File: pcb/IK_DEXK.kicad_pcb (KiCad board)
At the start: 2 copper layers, 70 x 76 mm, 11 parts, among them SW1 SW_Push, SW2 SW_Push, SW3 SW_Push, SW4 SW_Push, SW5 SW_Push, SW6 SW_Push, SW7 SW_Push, SW8 SW_Push, SW9 SW_Push, U1 MOUDLE-SEEEDUINO-XIAO, U2 ER_OLEDM0.91_1x-I2C

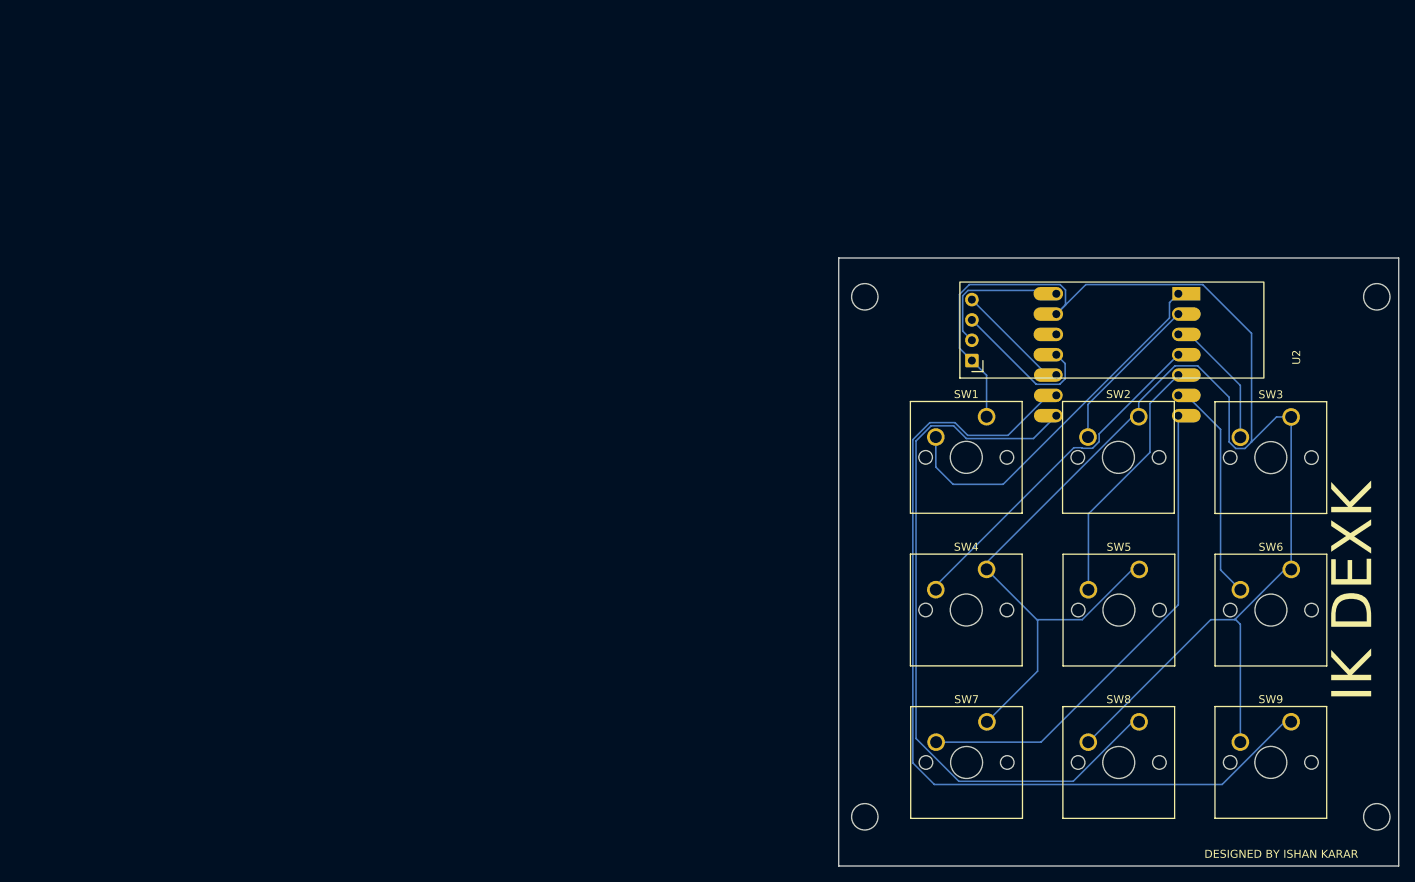
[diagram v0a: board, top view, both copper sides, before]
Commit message: everything
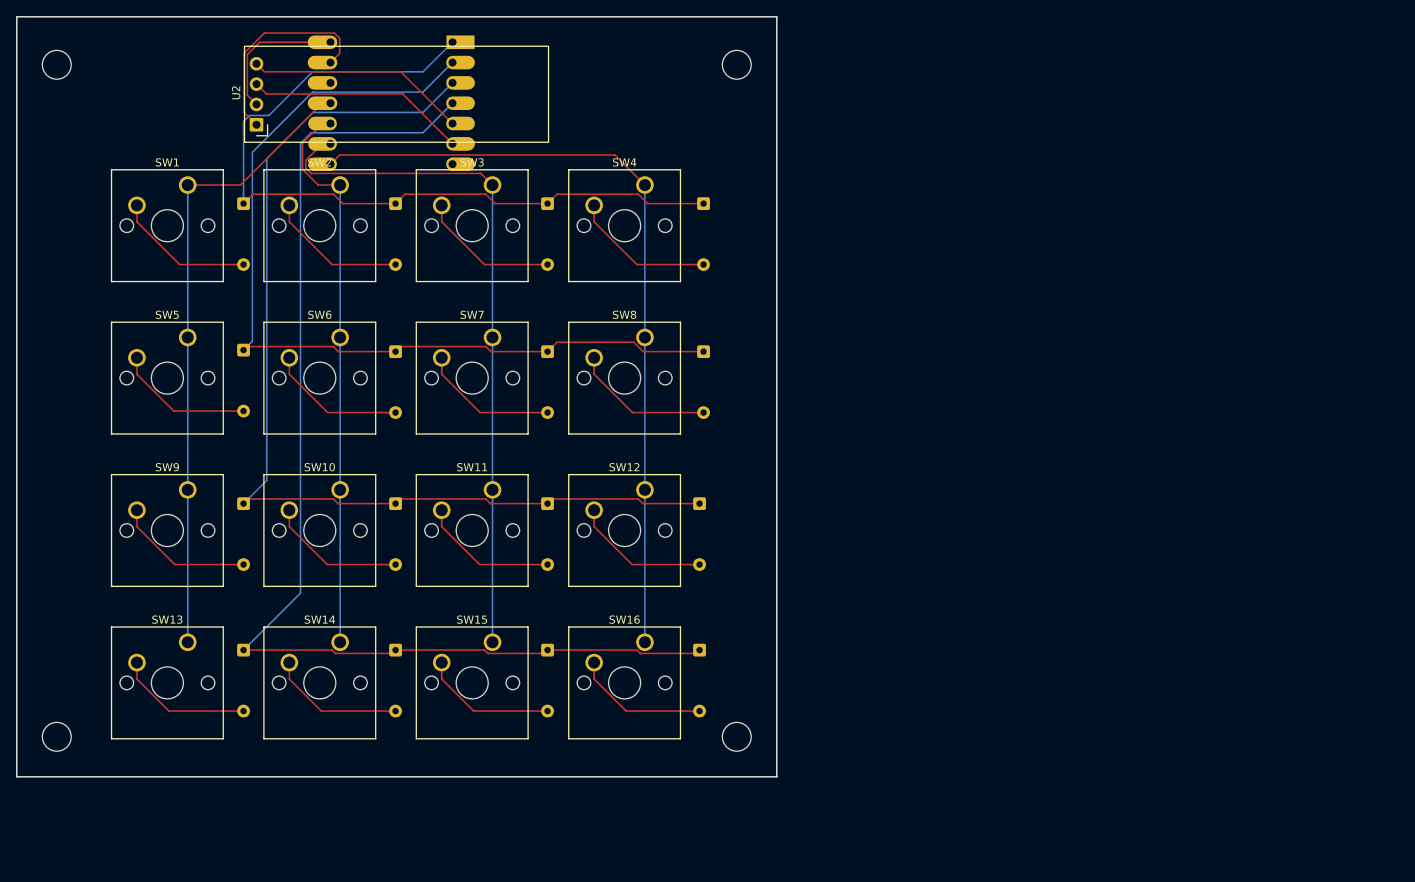
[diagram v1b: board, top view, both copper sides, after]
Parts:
- added D1: 1N4148, Diode_THT:D_DO-35_SOD27_P7.62mm_Horizontal, B.Cu at (28.3, 23.4)
- added D10: 1N4148, Diode_THT:D_DO-35_SOD27_P7.62mm_Horizontal, B.Cu at (47.3, 60.9)
- added D11: 1N4148, Diode_THT:D_DO-35_SOD27_P7.62mm_Horizontal, B.Cu at (66.3, 60.9)
- added D12: 1N4148, Diode_THT:D_DO-35_SOD27_P7.62mm_Horizontal, B.Cu at (85.3, 60.9)
- added D13: 1N4148, Diode_THT:D_DO-35_SOD27_P7.62mm_Horizontal, B.Cu at (28.3, 79.2)
- added D14: 1N4148, Diode_THT:D_DO-35_SOD27_P7.62mm_Horizontal, B.Cu at (47.3, 79.2)
- added D15: 1N4148, Diode_THT:D_DO-35_SOD27_P7.62mm_Horizontal, B.Cu at (66.3, 79.2)
- added D16: 1N4148, Diode_THT:D_DO-35_SOD27_P7.62mm_Horizontal, B.Cu at (85.3, 79.2)
- added D2: 1N4148, Diode_THT:D_DO-35_SOD27_P7.62mm_Horizontal, B.Cu at (47.3, 23.4)
- added D3: 1N4148, Diode_THT:D_DO-35_SOD27_P7.62mm_Horizontal, B.Cu at (66.3, 23.4)
- added D4: 1N4148, Diode_THT:D_DO-35_SOD27_P7.62mm_Horizontal, B.Cu at (85.8, 23.4)
- added D5: 1N4148, Diode_THT:D_DO-35_SOD27_P7.62mm_Horizontal, B.Cu at (28.3, 41.7)
- added D6: 1N4148, Diode_THT:D_DO-35_SOD27_P7.62mm_Horizontal, B.Cu at (47.3, 41.9)
- added D7: 1N4148, Diode_THT:D_DO-35_SOD27_P7.62mm_Horizontal, B.Cu at (66.3, 41.9)
- added D8: 1N4148, Diode_THT:D_DO-35_SOD27_P7.62mm_Horizontal, B.Cu at (85.8, 41.9)
- added D9: 1N4148, Diode_THT:D_DO-35_SOD27_P7.62mm_Horizontal, B.Cu at (28.3, 60.9)
- added SW10: SW_Push_45deg, Button_Switch_Keyboard:SW_Cherry_MX_1.00u_PCB, F.Cu at (40.4, 59.1)
- added SW11: SW_Push_45deg, Button_Switch_Keyboard:SW_Cherry_MX_1.00u_PCB, F.Cu at (59.5, 59.1)
- added SW12: SW_Push_45deg, Button_Switch_Keyboard:SW_Cherry_MX_1.00u_PCB, F.Cu at (78.5, 59.1)
- added SW13: SW_Push_45deg, Button_Switch_Keyboard:SW_Cherry_MX_1.00u_PCB, F.Cu at (21.4, 78.2)
- added SW14: SW_Push_45deg, Button_Switch_Keyboard:SW_Cherry_MX_1.00u_PCB, F.Cu at (40.4, 78.2)
- added SW15: SW_Push_45deg, Button_Switch_Keyboard:SW_Cherry_MX_1.00u_PCB, F.Cu at (59.5, 78.2)
- added SW16: SW_Push_45deg, Button_Switch_Keyboard:SW_Cherry_MX_1.00u_PCB, F.Cu at (78.5, 78.2)
- SW1, SW2, SW3, SW4, SW5, SW6, SW7, SW8, SW9: value SW_Push -> SW_Push_45deg
- moved SW9 140.9 mm to (21.4, 59.1)
- moved SW5 122.4 mm to (21.4, 40.1)
- moved SW6 122.4 mm to (40.4, 40.1)
- moved SW1 104.0 mm to (21.4, 21.0)
- moved SW3 104.0 mm to (59.5, 21.0)
- moved SW2 103.9 mm to (40.4, 21.0)
- moved U1 96.0 mm to (46.8, 10.8)
- moved U2 94.2 mm to (30.0, 13.5)
- moved SW7 78.3 mm to (59.5, 40.1)
- moved SW8 78.3 mm to (78.5, 40.1)
- moved SW4 64.3 mm to (78.5, 21.0)
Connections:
- net Net-(U1-5V) renamed VCC
- SW1 pad 1: GND -> /Column0
- SW1 pad 2: Net-(U1-PA02_A0_D0) -> Net-(D1-A)
- SW2 pad 1: GND -> /Column1
- SW2 pad 2: Net-(U1-PA4_A1_D1) -> Net-(D2-A)
- SW3 pad 1: GND -> /Column2
- SW3 pad 2: Net-(U1-PA10_A2_D2) -> Net-(D3-A)
- SW4 pad 1: GND -> /Column3
- SW4 pad 2: Net-(U1-PA11_A3_D3) -> Net-(D4-A)
- SW5 pad 1: GND -> /Column0
- SW5 pad 2: Net-(U1-PA8_A4_D4_SDA) -> Net-(D5-A)
- SW6 pad 1: GND -> /Column1
- SW6 pad 2: Net-(U1-PA9_A5_D5_SCL) -> Net-(D6-A)
- SW7 pad 1: GND -> /Column2
- SW7 pad 2: Net-(U1-PB08_A6_D6_TX) -> Net-(D7-A)
- SW8 pad 1: Net-(U1-PB09_A7_D7_RX) -> /Column3
- SW8 pad 2: GND -> Net-(D8-A)
- SW9 pad 1: Net-(U1-PA7_A8_D8_SCK) -> /Column0
- SW9 pad 2: GND -> Net-(D9-A)
- U1 pad 1: Net-(U1-PA02_A0_D0) -> /Row0
- U1 pad 10: Net-(U1-PA5_A9_D9_MISO) -> /Column1
- U1 pad 11: Net-(U1-PA6_A10_D10_MOSI) -> /Column0
- U1 pad 2: Net-(U1-PA4_A1_D1) -> /Row1
- U1 pad 3: Net-(U1-PA10_A2_D2) -> /Row2
- U1 pad 4: Net-(U1-PA11_A3_D3) -> /Row3
- U1 pad 7: Net-(U1-PB08_A6_D6_TX) -> unconnected-(U1-PB08_A6_D6_TX-Pad7)
- U1 pad 8: Net-(U1-PB09_A7_D7_RX) -> /Column3
- U1 pad 9: Net-(U1-PA7_A8_D8_SCK) -> /Column2
- U2 pad 3: Net-(U1-PA6_A10_D10_MOSI) -> Net-(U1-PA9_A5_D5_SCL)
- U2 pad 4: Net-(U1-PA5_A9_D9_MISO) -> Net-(U1-PA8_A4_D4_SDA)
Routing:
- net GND: track 244.3 -> 26.3 mm
- net /Row3: track 0.00 -> 145.4 mm
- net /Row2: track 0.00 -> 129.9 mm
- net /Row1: track 0.00 -> 114.3 mm
- net Net-(U1-PA7_A8_D8_SCK): track 113.6 -> 0.00 mm
- net /Row0: track 0.00 -> 100.9 mm
- net /Column3: track 0.00 -> 98.5 mm
- net Net-(U1-PB09_A7_D7_RX): track 90.5 -> 0.00 mm
- net /Column2: track 0.00 -> 86.3 mm
- net /Column0: track 0.00 -> 79.2 mm
- net /Column1: track 0.00 -> 70.4 mm
- net Net-(U1-PB08_A6_D6_TX): track 61.0 -> 0.00 mm
- net Net-(U1-PA02_A0_D0): track 45.9 -> 0.00 mm
- net Net-(U1-PA11_A3_D3): track 43.4 -> 0.00 mm
- net Net-(U1-PA4_A1_D1): track 20.0 -> 0.00 mm
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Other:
- board size 70 x 76 mm -> 95 x 95 mm
- board text removed: "DESIGNED BY ISHAN KARAR"
- board text removed: "IK DEXK"
